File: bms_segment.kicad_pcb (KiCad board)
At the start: 4 copper layers, 120 x 65 mm, 206 parts, among them J10 Conn_02x17_Counter_Clockwise, J3 Conn_02x10_Odd_Even, J4 Conn_02x10_Odd_Even, J5 Conn_01x04, J6 Conn_01x04, J7 Conn_01x06, Q1 IRLML0060, Q10 IRLML0060, Q11 IRLML0060, Q12 IRLML0060, Q13 IRLML0060, Q14 IRLML0060, Q15 IRLML0060, Q16 IRLML0060, Q17 BSS84, Q2 IRLML0060, Q3 IRLML0060, Q4 IRLML0060, Q5 IRLML0060, Q6 IRLML0060, Q7 IRLML0060, Q8 IRLML0060, Q9 IRLML0060, SW1 SW_Push, U1 LMR516xx, U2 MAX14921, U3 MAX11163, U4 REF61xx, U5 STM32F103C8Tx, U6 ADuM1252, U7 74LV4051A, U8 74LV4051A, U9 74LV4051A

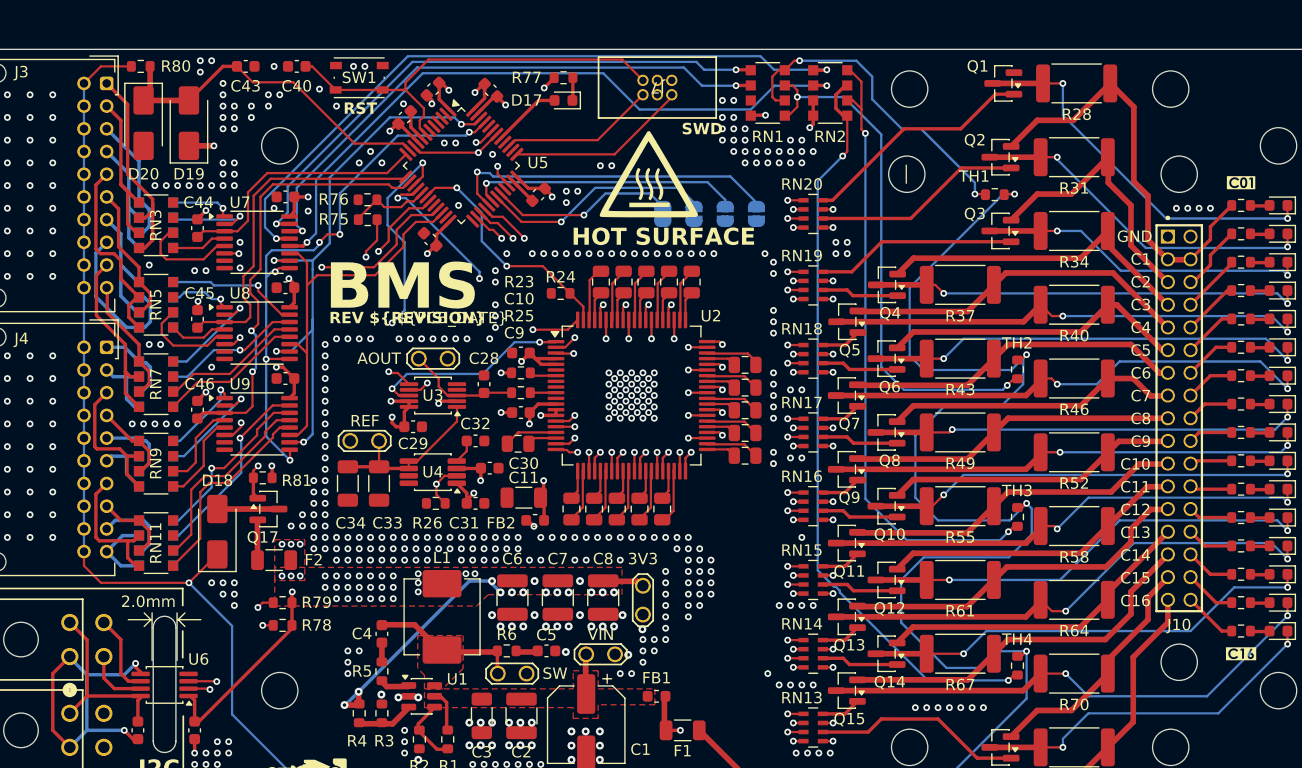
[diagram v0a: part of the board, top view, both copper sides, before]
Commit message: pcb: Run track cleanup
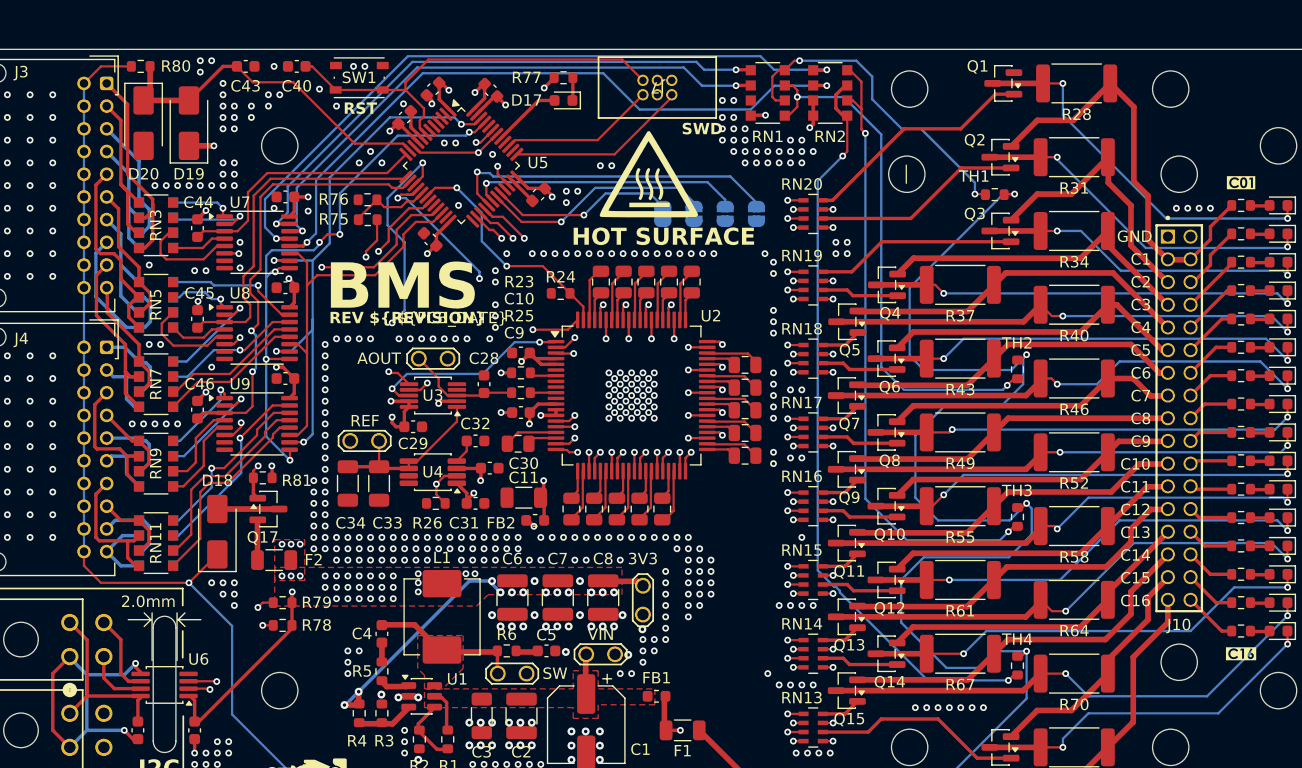
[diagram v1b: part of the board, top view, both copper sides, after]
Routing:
- net +3V3: track 98.8 -> 96.8 mm, vias 63 -> 60
- net TAP3: track 67.4 -> 66.0 mm
- net TAP15: track 63.8 -> 62.5 mm
- net /Thermistor Sampling/Thermistors/PWR: track 251.3 -> 250.1 mm
- net Net-(U2-LDOIN): track 11.4 -> 10.6 mm
- net /Thermistor Sampling/RAIL: track 31.0 -> 30.2 mm
- net GND: track 26.7 -> 26.0 mm
- net /Thermistor Sampling/Thermistors/Network/IN_2: track 46.6 -> 45.9 mm
- net TAP13: track 69.1 -> 68.4 mm
- net /Thermistor Sampling/Thermistors/Network1/IN_1: track 55.5 -> 54.9 mm
- net /Thermistor Sampling/Thermistors/Network9/IN_1: track 6.82 -> 6.28 mm
- net Net-(D10-K): track 38.6 -> 38.1 mm
